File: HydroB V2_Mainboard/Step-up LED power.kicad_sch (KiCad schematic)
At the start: 18 parts, among them Q1 S8050

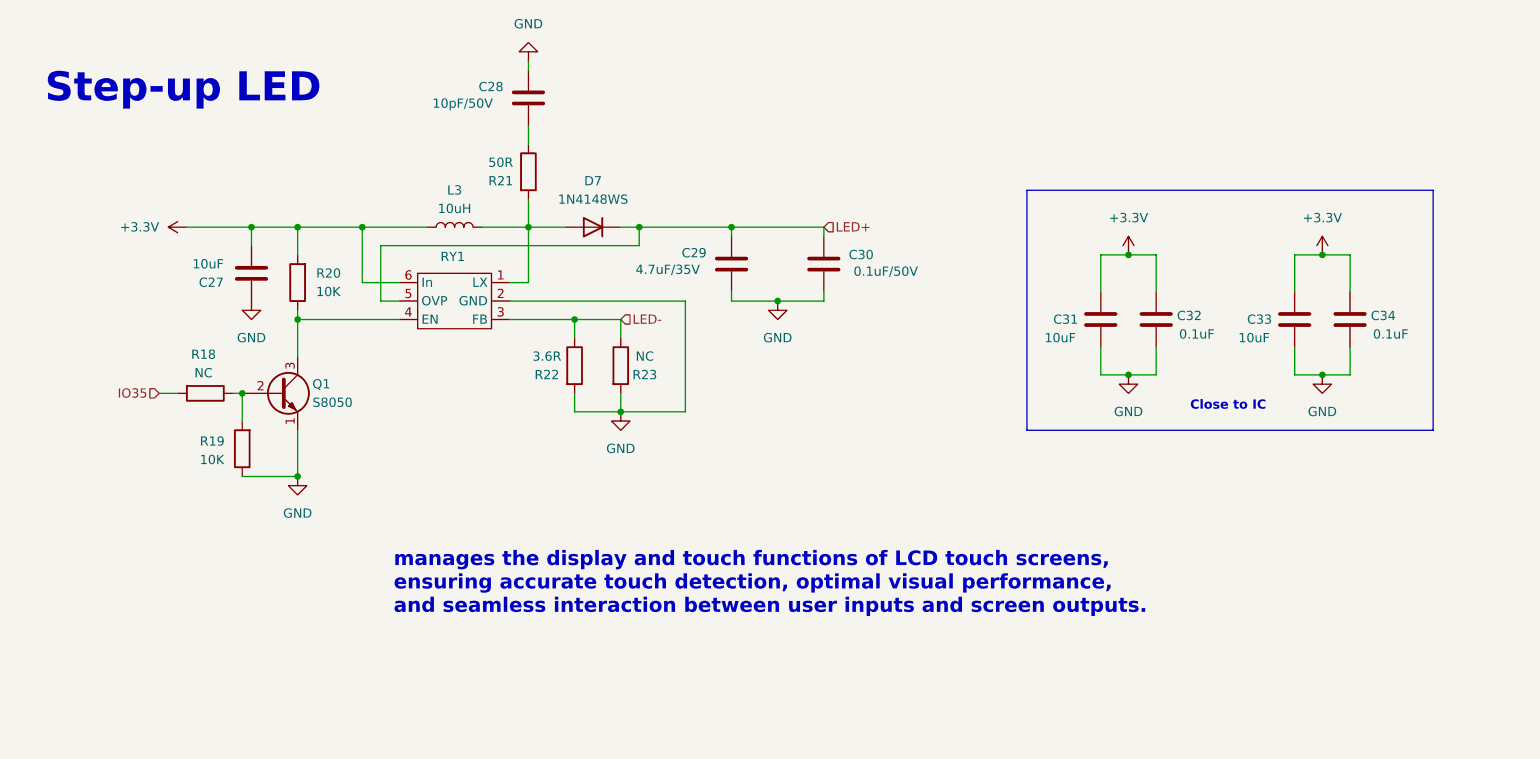
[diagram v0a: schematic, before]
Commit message: Schematic mainboard update
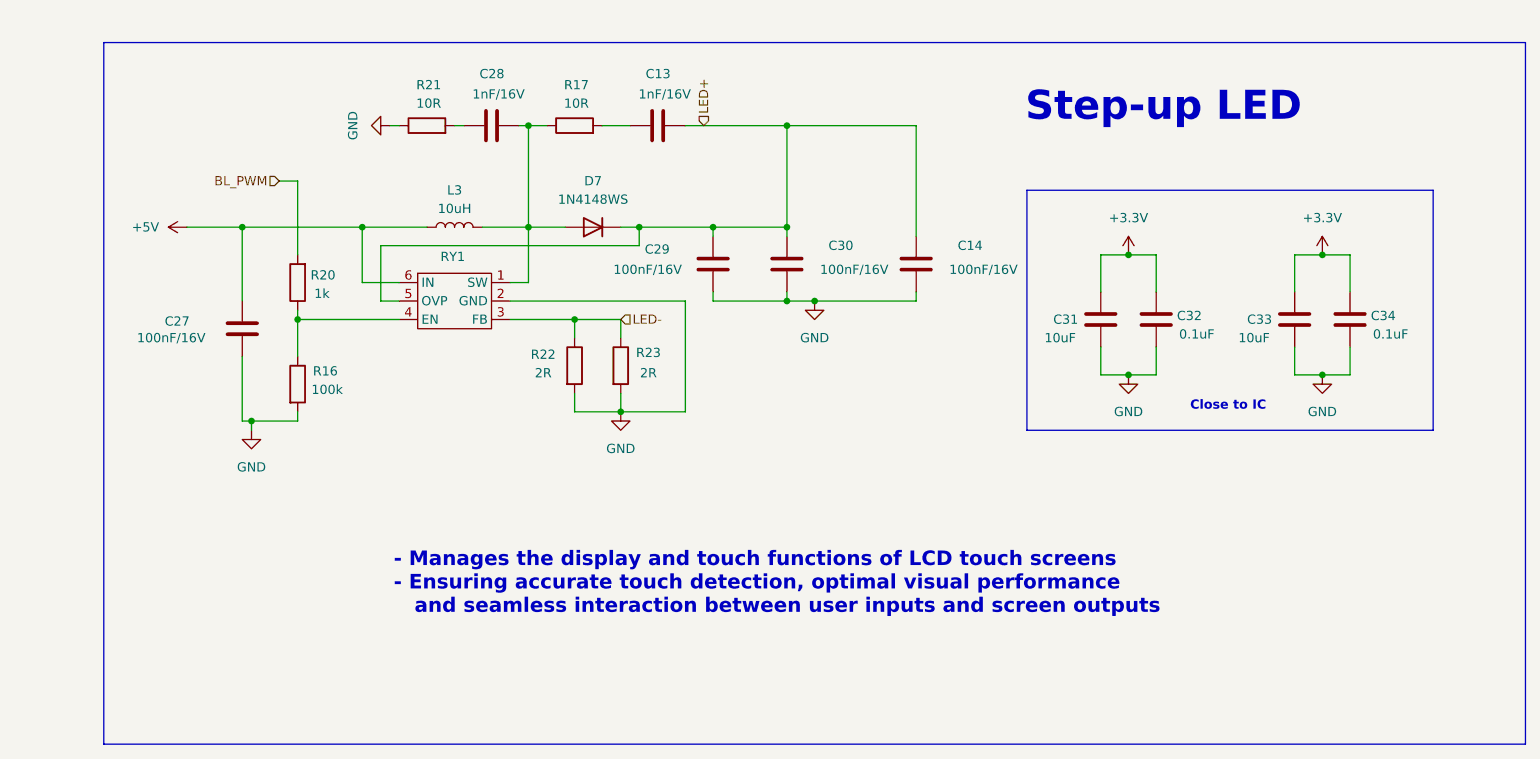
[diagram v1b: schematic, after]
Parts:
- removed Q1: S8050, Package_TO_SOT_THT:TO-92_Inline, symbol Transistor_BJT:S8050
- removed R18: NC, Resistor_SMD:R_0603_1608Metric, symbol Device:R
- removed R19: 10K, Resistor_SMD:R_0603_1608Metric, symbol Device:R
- added C13: 1nF/16V, Capacitor_SMD:C_0805_2012Metric, symbol Device:C
- added C14: 100nF/16V, Capacitor_SMD:C_0603_1608Metric, symbol Device:C
- added R16: 100k, Resistor_SMD:R_0603_1608Metric, symbol Device:R
- added R17: 10R, Resistor_SMD:R_0603_1608Metric, symbol Device:R
- C27: value 10uF -> 100nF/16V
- C28: value 10pF/50V -> 1nF/16V; footprint Capacitor_SMD:C_0805_2012Metric -> Capacitor_SMD:C_0603_1608Metric
- C29: value 4.7uF/35V -> 100nF/16V; footprint Capacitor_Tantalum_SMD:CP_EIA-7343-43_Kemet-X_Pad2.25x2.55mm_HandSolder -> Capacitor_Tantalum_SMD:CP_EIA-6032-28_Kemet-C
- C30: value 0.1uF/50V -> 100nF/16V; footprint Capacitor_Tantalum_SMD:CP_EIA-7343-43_Kemet-X_Pad2.25x2.55mm_HandSolder -> Capacitor_SMD:C_0603_1608Metric
- L3: footprint Inductor_SMD:L_Bourns_SRR1260 -> Inductor_SMD:L_Bourns_SRP5030T
- R20: value 10K -> 1k
- R21: value 50R -> 10R
- R22: value 3.6R -> 2R
- R23: value NC -> 2R
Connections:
- net +3.3V: no longer C27.2, L3.1, R20.2, RY1.6 (In)
- net GND: now also R21.1, C14.1, R16.2; no longer C28.2
- net LED+: now also C13.1, C14.2
- net at R20.1, RY1.4 (EN): now also R16.1
- net at D7.2 (A), L3.2, RY1.1 (SW): now also C28.1, R17.1; no longer R21.2
- new net: C13.2, R17.2
- new net: C28.2, R21.2
- new net +5V: C27.2, L3.1, RY1.6 (IN)
- new net BL_PWM: R20.2
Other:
- note added: "- Manages the display and touch functions of LCD touch screens - Ensuring accurate touch detection, optimal visual performance and seamless interaction between user inputs and screen outputs"
- note removed: "manages the display and touch functions of LCD touch screens, ensuring accurate touch detection, optimal visual performance, and seamless interaction between user inputs and screen outputs."
- moved on the sheet: C27, C28, C29, C30, R21
